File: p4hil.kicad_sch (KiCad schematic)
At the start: 8 parts, among them J14 Conn_01x04, SW1 SW_Push, SW2 SW_Push, U5 PI4IOE5V9535ZDEX

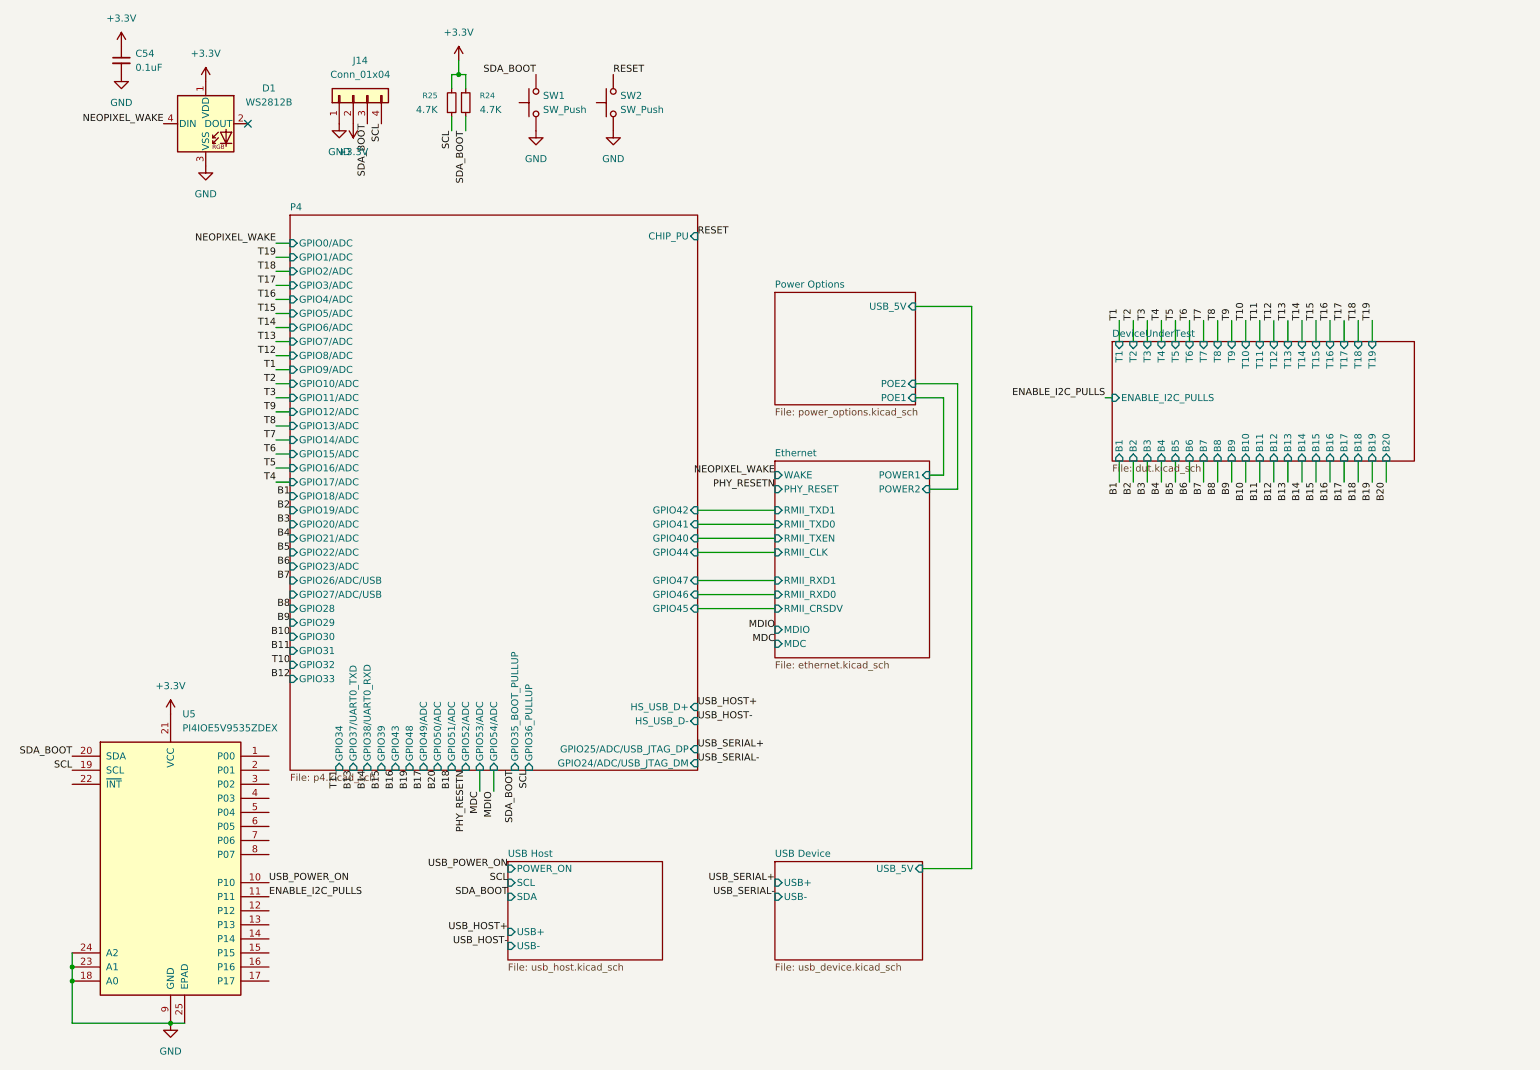
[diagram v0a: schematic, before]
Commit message: clean drc
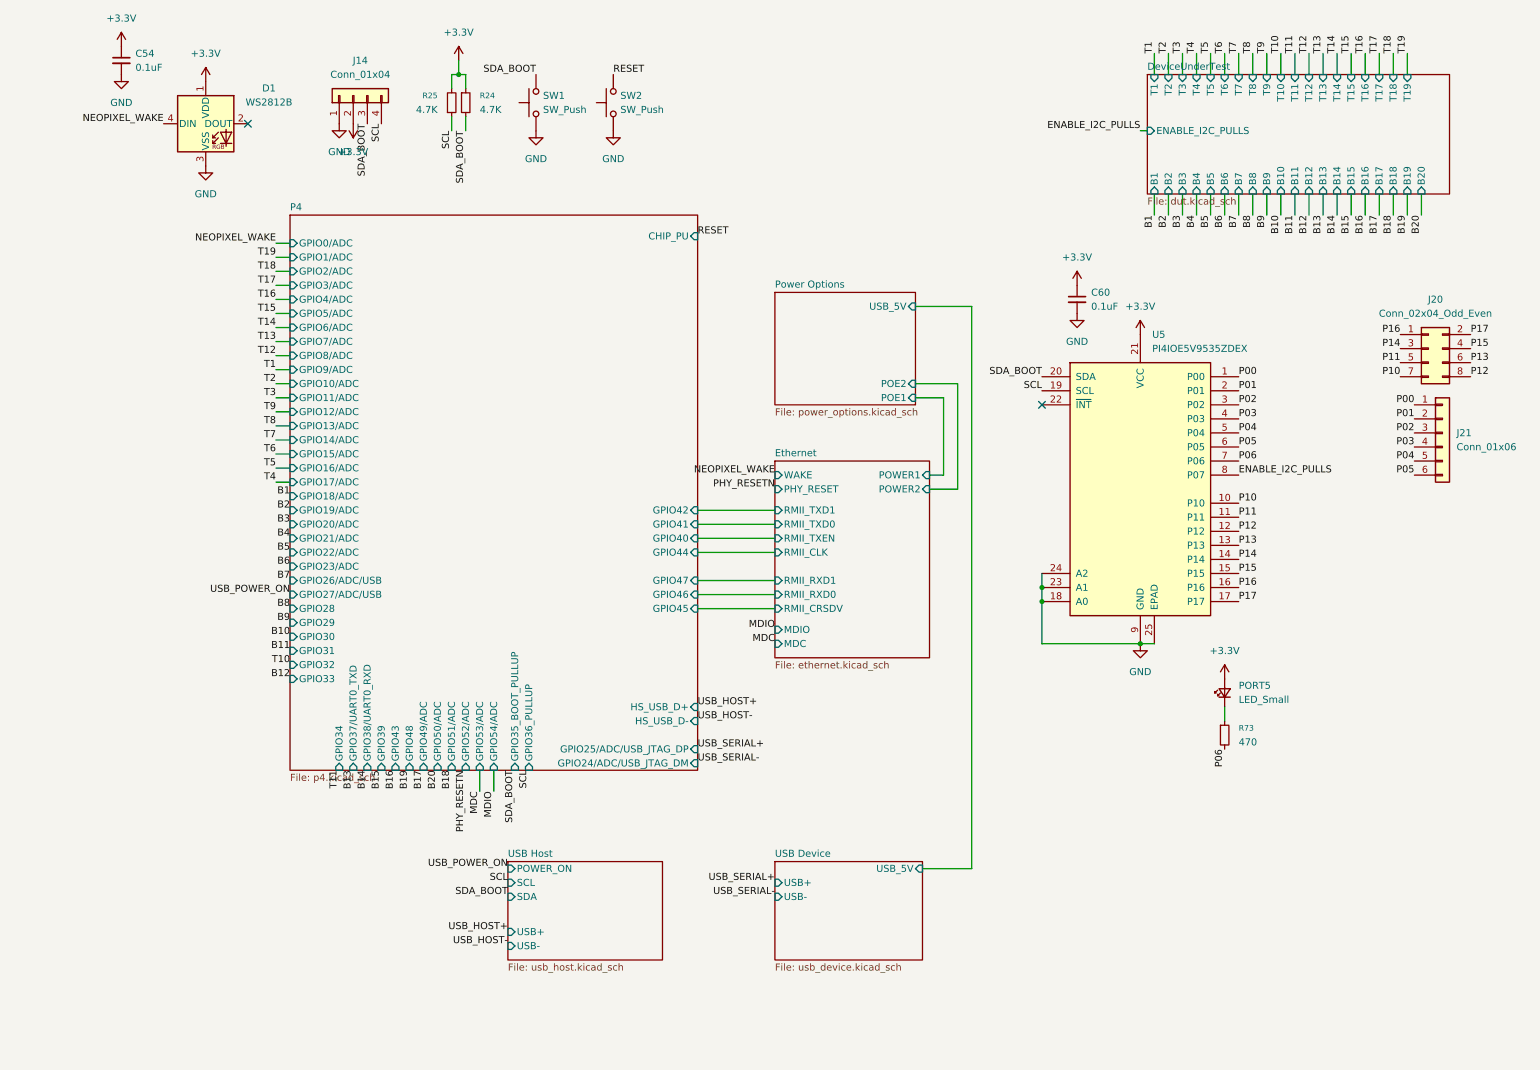
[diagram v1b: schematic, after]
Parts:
- added C60: 0.1uF, Capacitor_SMD:C_0402_1005Metric, symbol Device:C_Small
- added J20: Conn_02x04_Odd_Even, Connector_PinHeader_2.54mm:PinHeader_2x04_P2.54mm_Vertical, symbol Connector_Generic:Conn_02x04_Odd_Even
- added J21: Conn_01x06, Connector_PinHeader_2.54mm:PinHeader_1x06_P2.54mm_Vertical, symbol Connector_Generic:Conn_01x06
- added PORT5: LED_Small, LED_SMD:LED_0603_1608Metric, symbol Device:LED_Small
- added R73: 470, Resistor_SMD:R_0402_1005Metric, symbol Device:R_Small
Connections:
- net +3.3V: now also C60.1, PORT5.2 (A)
- net ENABLE_I2C_PULLS: now also U5.8 (P07); no longer U5.11 (P11)
- net GND: now also C60.2
- net USB_POWER_ON: no longer U5.10 (P10)
- net P00: now reaches U5.1 (P00)
- net P00: now also J21.1 (Pin_1)
- net P12: now reaches U5.12 (P12)
- net P12: now also J20.8 (Pin_8)
- net P13: now reaches U5.13 (P13)
- net P13: now also J20.6 (Pin_6)
- net P14: now reaches U5.14 (P14)
- net P14: now also J20.3 (Pin_3)
- net P15: now reaches U5.15 (P15)
- net P15: now also J20.4 (Pin_4)
- net P16: now reaches U5.16 (P16)
- net P16: now also J20.1 (Pin_1)
- net P17: now reaches U5.17 (P17)
- net P17: now also J20.2 (Pin_2)
- net P01: now reaches U5.2 (P01)
- net P01: now also J21.2 (Pin_2)
- net P02: now reaches U5.3 (P02)
- net P02: now also J21.3 (Pin_3)
- net P03: now reaches U5.4 (P03)
- net P03: now also J21.4 (Pin_4)
- net P04: now reaches U5.5 (P04)
- net P04: now also J21.5 (Pin_5)
- net P05: now reaches U5.6 (P05)
- net P05: now also J21.6 (Pin_6)
- net P06: now reaches U5.7 (P06)
- net P06: now also R73.2
- new net: PORT5.1 (K), R73.1
- new net P10: J20.7 (Pin_7), U5.10 (P10)
- new net P11: J20.5 (Pin_5), U5.11 (P11)
- no-connect marks 1 -> 2
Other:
- moved on the sheet: U5
